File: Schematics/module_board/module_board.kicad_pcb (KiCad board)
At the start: 2 copper layers, 30 x 30 mm, 26 parts, among them J1 Conn_01x04_Male, J10 Conn_01x02_Male, J2 Conn_01x10_Male, J5 Conn_01x06_Male, J9 Conn_01x02_Male, U1 RP2040, U2 W25Q16JVSSIQ, Y1 ABLS-12.000MHZ-B4-T

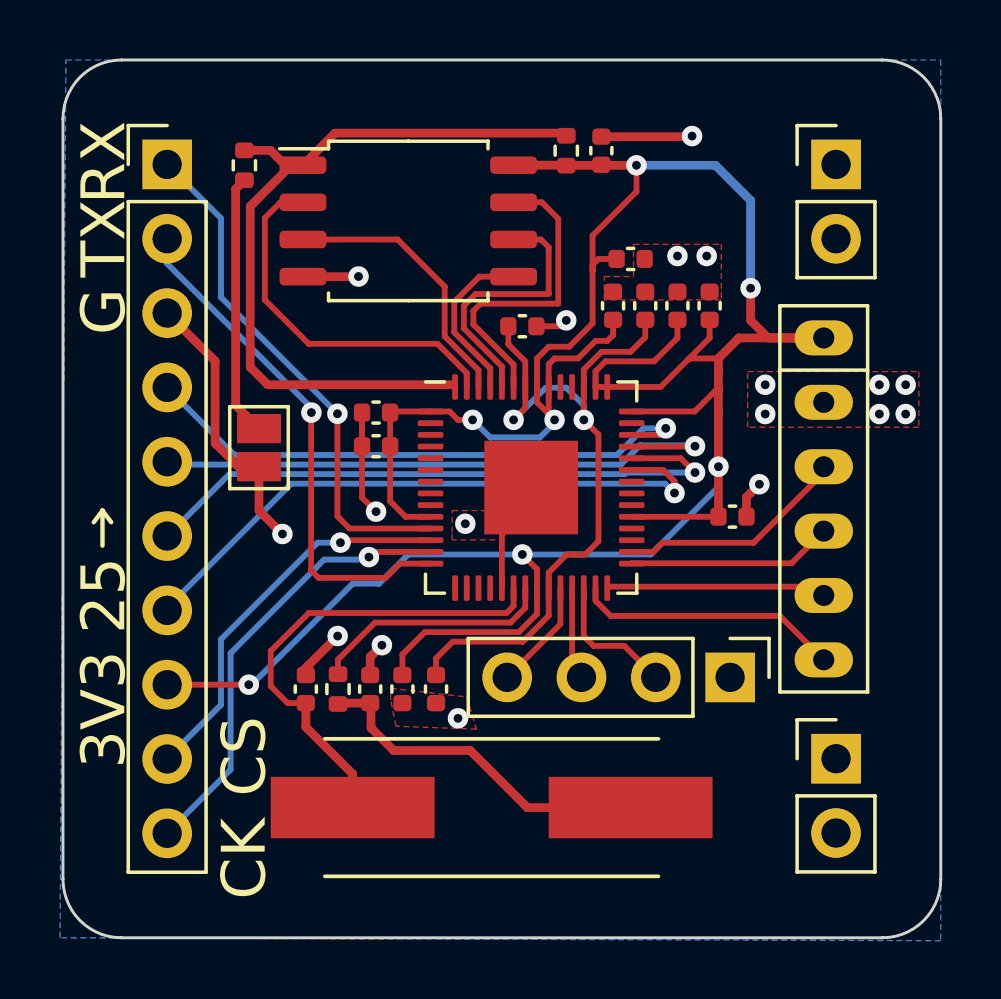
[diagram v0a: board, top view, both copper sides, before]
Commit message: Final improvements
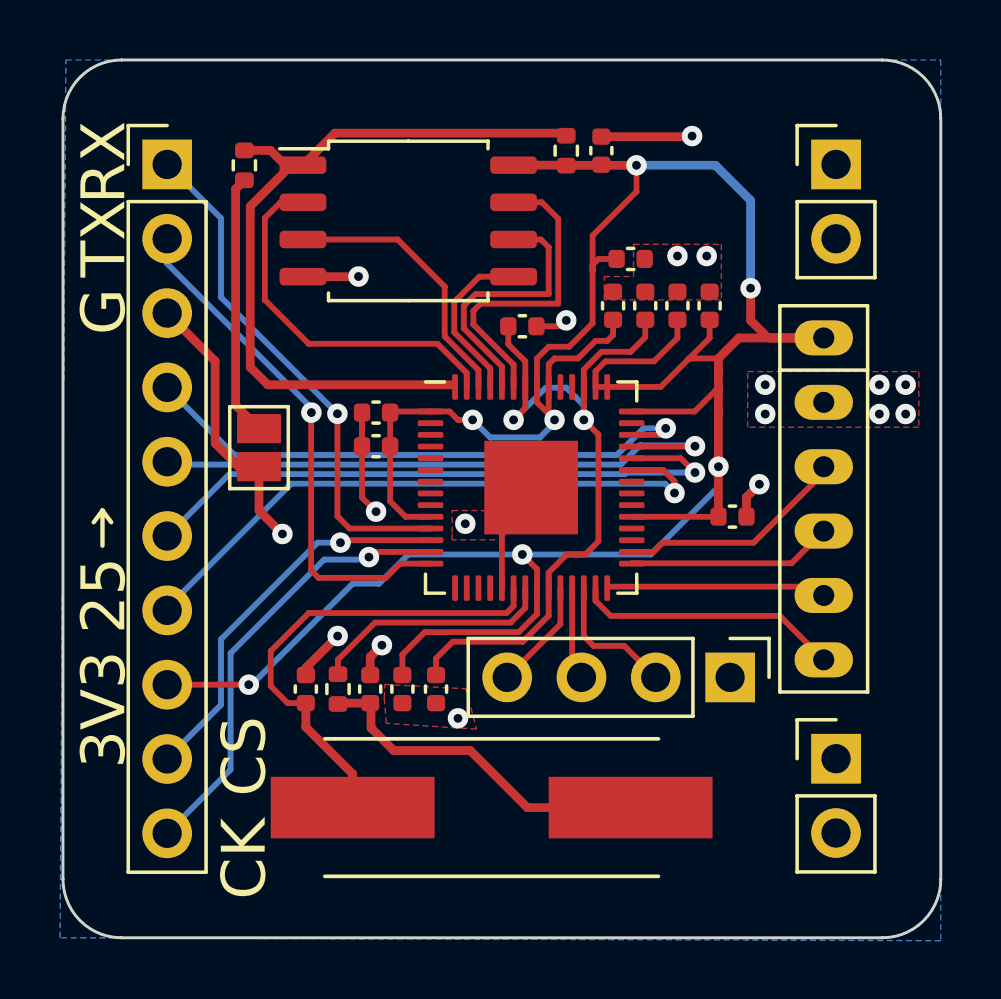
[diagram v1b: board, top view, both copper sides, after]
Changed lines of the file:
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@@
       (pts
         (xy 159.130238 97.868975)
-        (xy 156.381832 97.768975)
-        (xy 156.2 96.869635)
-        (xy 156.2 96.469635)
-        (xy 158.8 96.769635)
+        (xy 156.05 97.67)
+        (xy 155.98 96.81)
+        (xy 156 96.34)
+        (xy 158.77 96.49)
       )
     )
